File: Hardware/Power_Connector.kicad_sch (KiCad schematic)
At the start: 3 parts, among them J401 AMASS XT60 Male, J402 AMASS XT60 Female

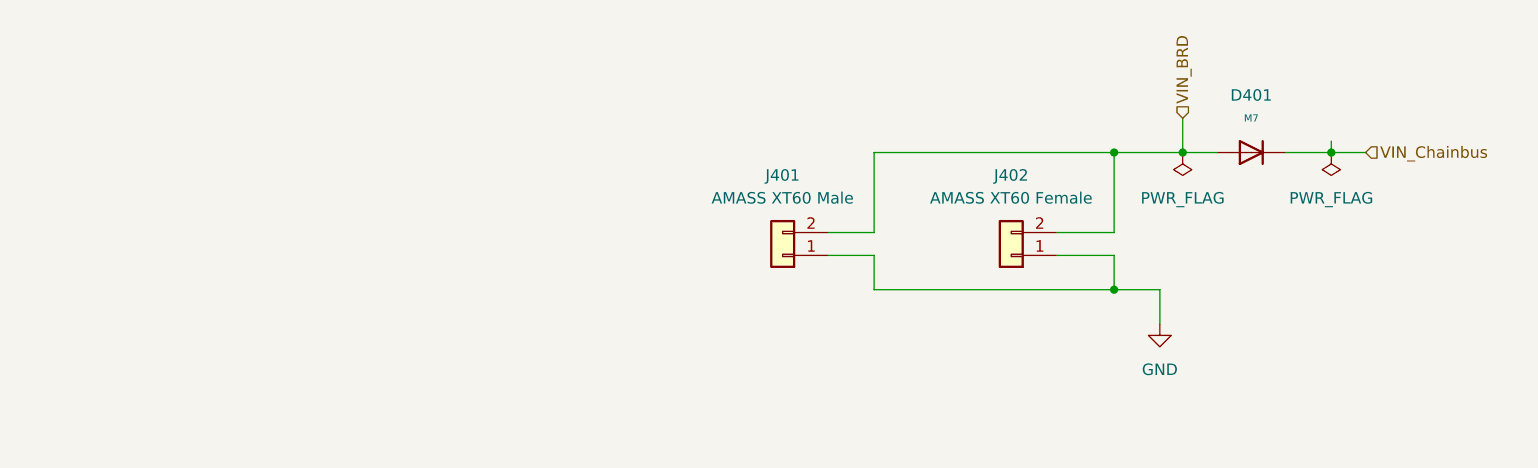
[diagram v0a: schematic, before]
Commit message: working commit
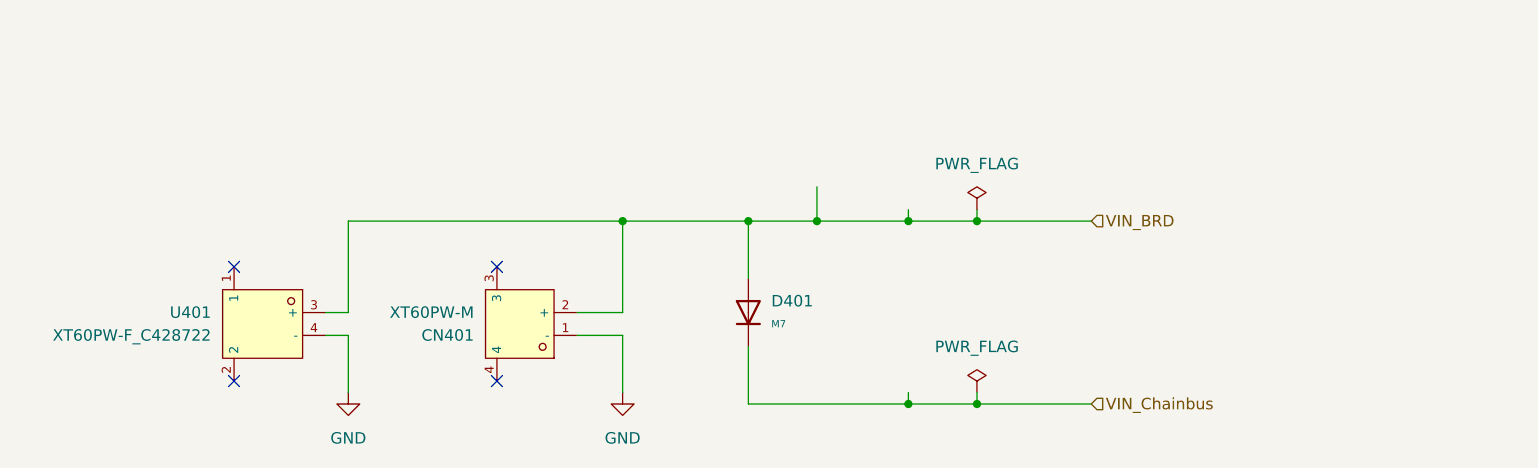
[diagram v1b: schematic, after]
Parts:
- removed J401: AMASS XT60 Male, XT60:AMASS_XT60PW-M_1x02_P7.20mm_Horizontal, symbol Connector_Generic:Conn_01x02
- removed J402: AMASS XT60 Female, XT60:AMASS_XT60PW-F_1x02_P7.20mm_Horizontal, symbol Connector_Generic:Conn_01x02
- added CN401: XT60PW-M, lcsc_footprints:C98732_CONN-TH_XT60PW-M, symbol lcsc_imported:XT60PW-M
- added U401: XT60PW-F_C428722, lcsc_footprints:C428722_TH_2P-XT60PW-F, symbol lcsc_imported:XT60PW-F_C428722
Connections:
- net GND: now also CN401.1 (-), U401.4 (-)
- net VIN_BRD: now also CN401.2 (+), U401.3 (+)
- no-connect marks 0 -> 4
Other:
- title: MMS3 Hat template small (Change Me) -> MMS3_hat_motor_high_power
